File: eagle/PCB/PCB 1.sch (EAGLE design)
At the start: 36 parts

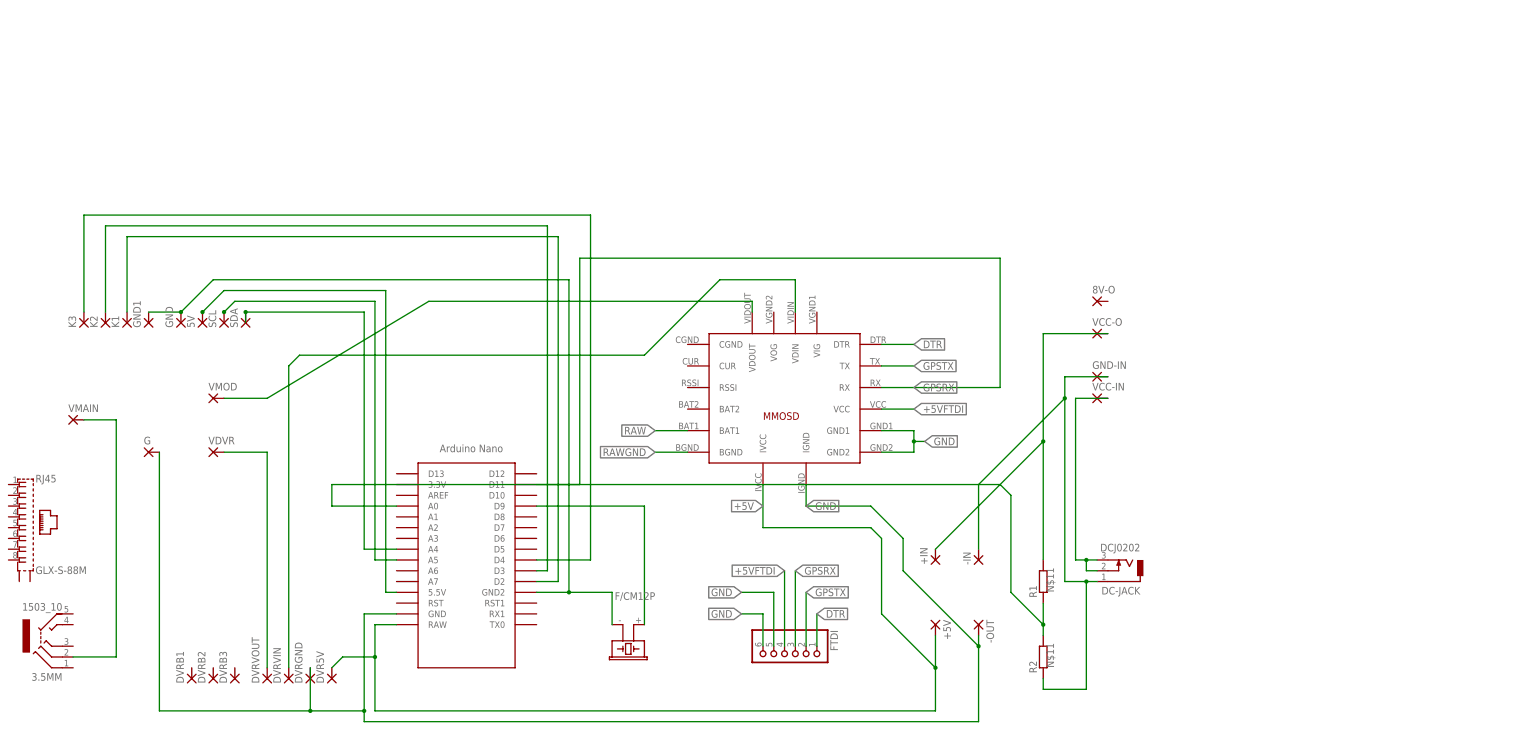
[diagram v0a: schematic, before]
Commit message: PCB work
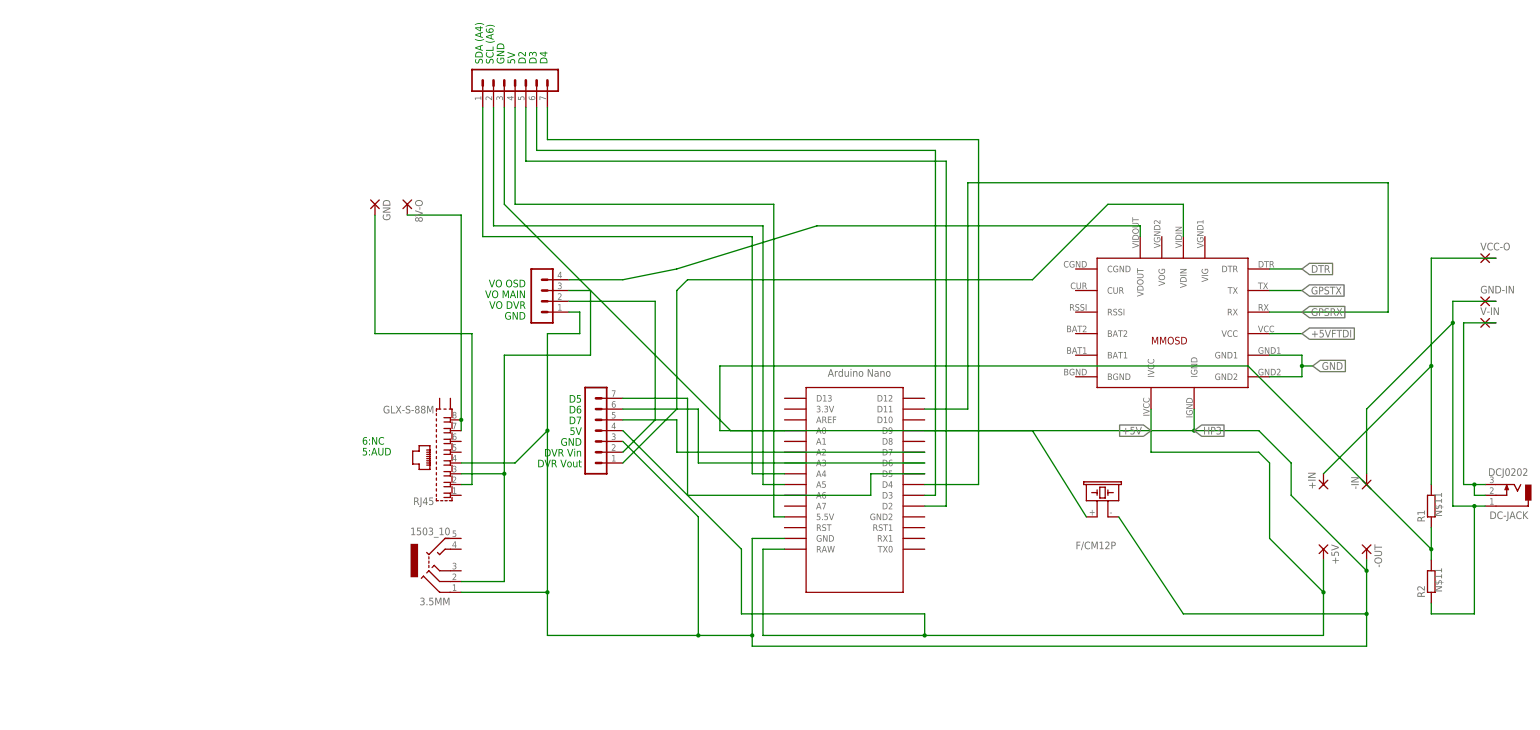
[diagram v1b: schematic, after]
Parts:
- removed 5V, DVR5V, DVRB1, DVRB2, DVRB3, DVRGND, DVRVIN, DVRVOUT, G, GND1, K1, K2, K3, SCL, SDA, VDVR, VMAIN, VMOD: (no value), wirepad:SMD2
- removed FTDI: (no value), pinhead:PINHD-1X6
- removed VCC-IN: (no value), wirepad:2,54/1,1
- added IO1, IO2: (no value), con-lstb:MA07-1
- added IO3: (no value), con-lstb:MA04-1
- added V-IN: (no value), wirepad:2,54/1,1
- GND: device wirepad:SMD2 -> wirepad:2,54/1,1
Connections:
- removed net N$1: ADRUINO-NANO.GND2, BUZZ.2, GND.P, GND1.P
- removed net N$3 (its old number): ADRUINO-NANO.A5, SCL.P
- removed net RAW: MINIMOSD.BAT1
- removed net RAWGND: MINIMOSD.BGND
- new net HP1: ADRUINO-NANO.A4, IO2.1
- new net HP2: ADRUINO-NANO.A5, IO2.2
- new net HP3: -OUT.P, 3.5MM.1, ADRUINO-NANO.GND, BUZZ.2, IO1.3, IO2.3, IO3.1, MINIMOSD.IGND, RJ45.4
- new net HP5: ADRUINO-NANO.D2, IO2.5
- new net HP6: ADRUINO-NANO.D3, IO2.6
- new net HP7: ADRUINO-NANO.D4, IO2.7
- new net N$6: 8V-O.P, RJ45.7, RJ45.8
- net +5V: now also IO1.4; no longer DVR5V.P
- net +5VFTDI: no longer FTDI.4
- net DTR: no longer FTDI.1
- net GND: no longer -OUT.P, ADRUINO-NANO.GND, DVRGND.P, FTDI.5, FTDI.6, G.P, MINIMOSD.IGND
- net GPSRX: no longer FTDI.3
- net GPSTX: no longer FTDI.2
- net N$14: now also IO1.2, IO3.2; no longer DVRVOUT.P, VDVR.P
- net N$15: now also IO3.3, RJ45.3; no longer VMAIN.P
- net N$2: now also IO2.4; no longer 5V.P
- net N$4: now also ADRUINO-NANO.D5, IO1.7; no longer ADRUINO-NANO.A4, SDA.P
- net N$5: now also V-IN.P; no longer VCC-IN.P
- net N$7: now also GND.P, RJ45.2; no longer ADRUINO-NANO.D2, K1.P
- net N$8: now also ADRUINO-NANO.D6, IO1.6; no longer ADRUINO-NANO.D3, K2.P
- net N$9: now also ADRUINO-NANO.D7, IO1.5; no longer ADRUINO-NANO.D4, K3.P
- net VIDIN: now also IO1.1; no longer DVRVIN.P
- net VIDOUT: now also IO3.4; no longer VMOD.P
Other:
- note added: "5:AUD"
- note added: "5V"
- note added: "6:NC"
- note added: "D2"
- note added: "D3"
- note added: "D4"
- note added: "D5"
- note added: "D6"
- note added: "D7"
- note added: "DVR Vin"
- note added: "DVR Vout"
- note added: "GND"
- note added: "SCL (A6)"
- note added: "SDA (A4)"
- note added: "VO DVR"
- note added: "VO MAIN"
- note added: "VO OSD"
- moved on the sheet: +5V, +IN, -IN, -OUT, 3.5MM, 8V-O, DC-JACK, GND, GND-IN, R1, R2, RJ45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
